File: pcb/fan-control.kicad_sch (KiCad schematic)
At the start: 23 parts, among them J1 USB_C_Receptacle_USB2.0_14P, J2 USB_C_Receptacle_USB2.0_14P, Q1 BSS138, SW1 SW_Push, U1 ESP32-C6-WROOM-1-N8

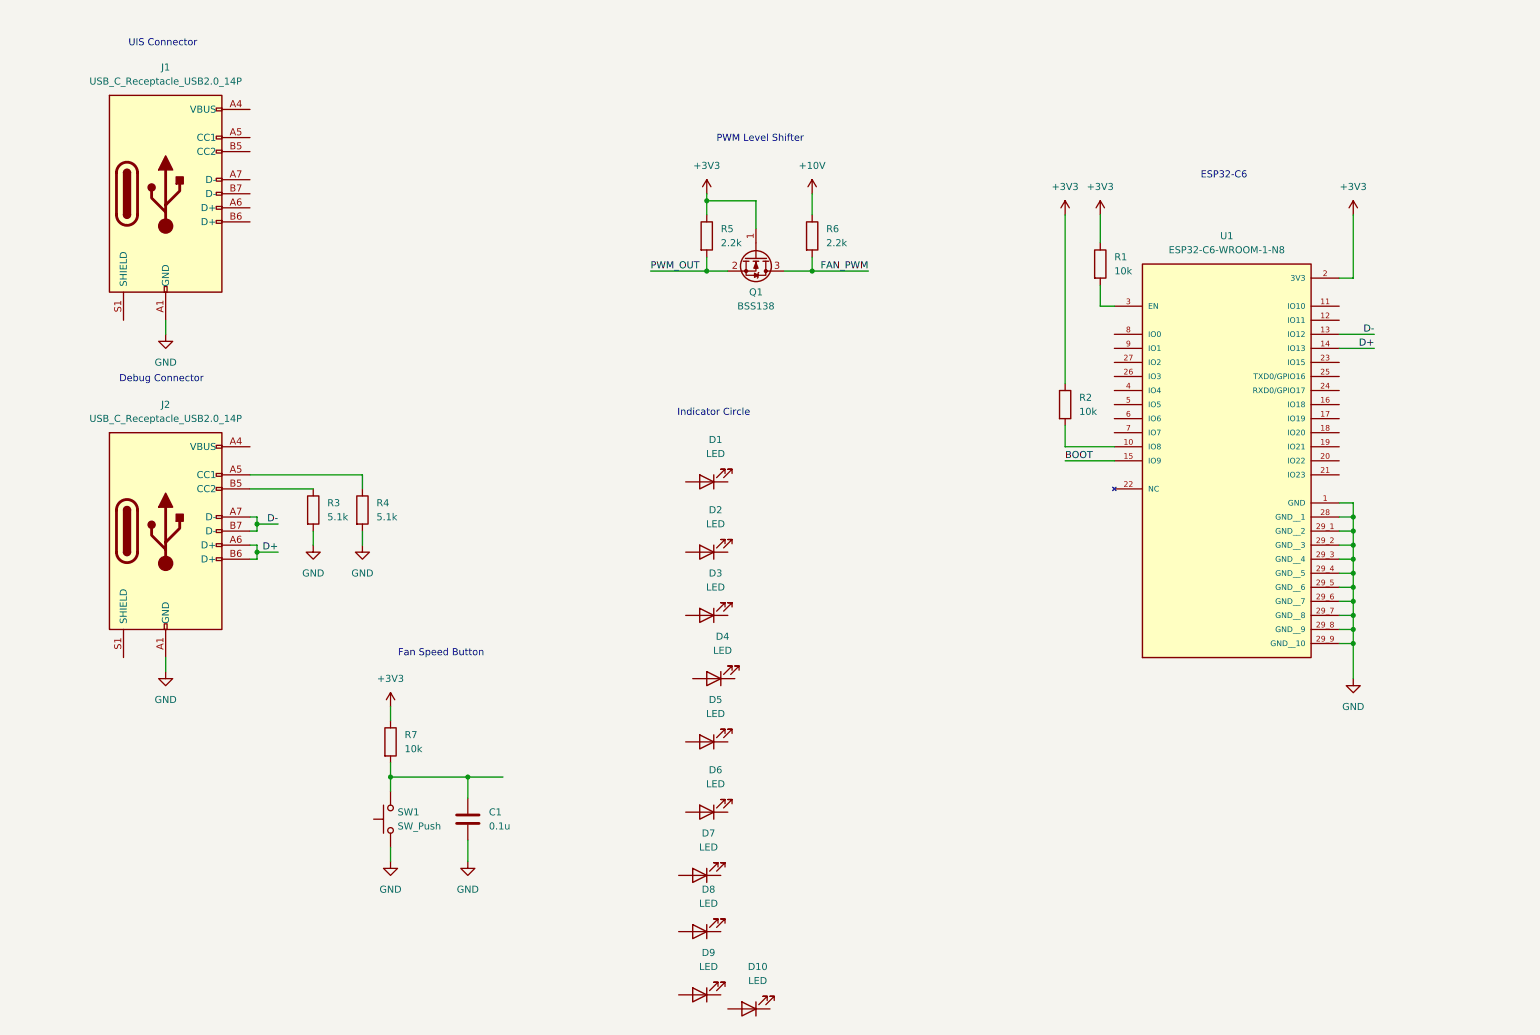
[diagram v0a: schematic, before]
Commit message: schematic
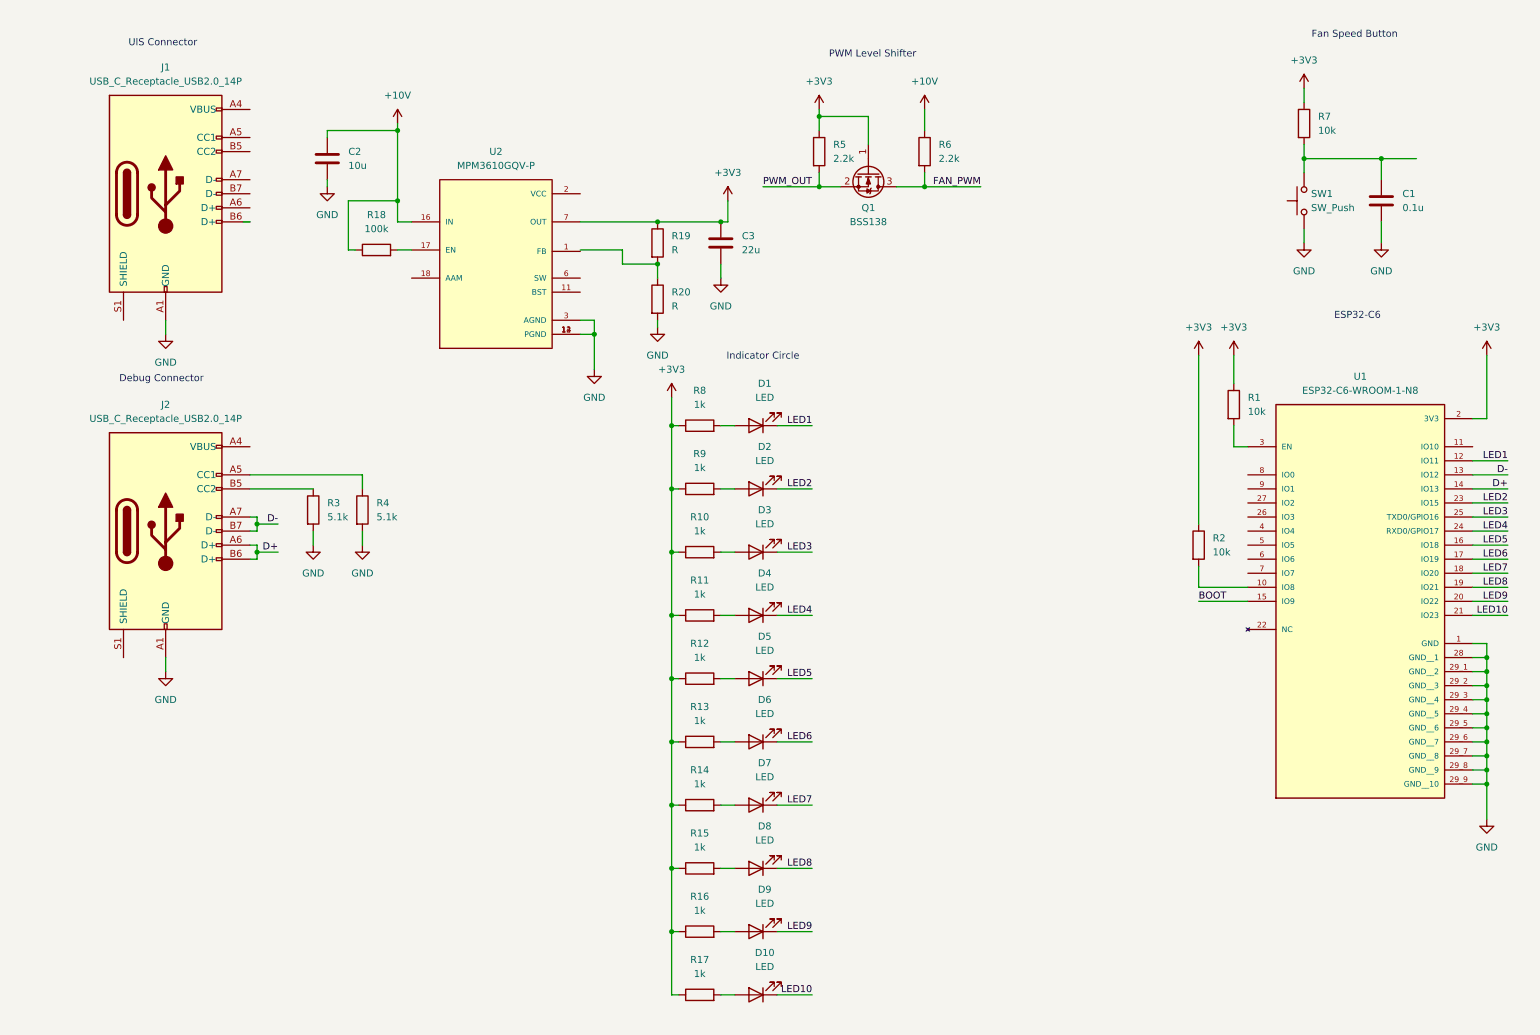
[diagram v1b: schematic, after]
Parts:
- added C2: 10u, symbol Device:C
- added C3: 22u, symbol Device:C
- added R10, R11, R12, R13, R14, R15, R16, R17, R8, R9: 1k, symbol Device:R
- added R18: 100k, symbol Device:R
- added R19, R20: R, symbol Device:R
- added U2: MPM3610GQV-P, MPM3610GQV-P:CONV_MPM3610GQV-P, symbol MPM3610GQV-P:MPM3610GQV-P
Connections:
- net +10V: now also C2.1, R18.1, U2.16 (IN)
- net +3V3: now also C3.1, R10.1, R11.1, R12.1, R13.1, R14.1, R15.1, R16.1, R17.1, R19.1, R8.1, R9.1, U2.7 (OUT)
- net GND: now also C2.2, C3.2, R20.2, U2.12 (PGND), U2.13 (PGND), U2.14 (PGND), U2.3 (AGND)
- net LED1: now reaches D1.1 (K)
- net LED1: now also U1.12 (IO11)
- net at D1.2 (A): now also R8.2
- net LED10: now reaches D10.1 (K)
- net LED10: now also U1.21 (IO23)
- net at D10.2 (A): now also R17.2
- net LED3: now reaches D3.1 (K)
- net LED3: now also U1.25 (TXD0/GPIO16)
- net at D3.2 (A): now also R10.2
- net LED7: now reaches D7.1 (K)
- net LED7: now also U1.18 (IO20)
- net at D7.2 (A): now also R14.2
- net LED8: now reaches D8.1 (K)
- net LED8: now also U1.19 (IO21)
- net at D8.2 (A): now also R15.2
- net LED5: now reaches U1.16 (IO18)
- net LED5: now also D5.1 (K)
- net LED6: now reaches U1.17 (IO19)
- net LED6: now also D6.1 (K)
- net LED9: now reaches U1.20 (IO22)
- net LED9: now also D9.1 (K)
- net LED2: now reaches U1.23 (IO15)
- net LED2: now also D2.1 (K)
- net LED4: now reaches U1.24 (RXD0/GPIO17)
- net LED4: now also D4.1 (K)
- net at D5.2 (A): now also R12.2
- net at D4.2 (A): now also R11.2
- net at D9.2 (A): now also R16.2
- net at D6.2 (A): now also R13.2
- net at D2.2 (A): now also R9.2
- new net: R18.2, U2.17 (EN)
- new net: R19.2, R20.1
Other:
- moved on the sheet: C1, D1, D10, D2, D3, D4, D5, D6, D7, D8, D9, Q1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

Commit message: More sch
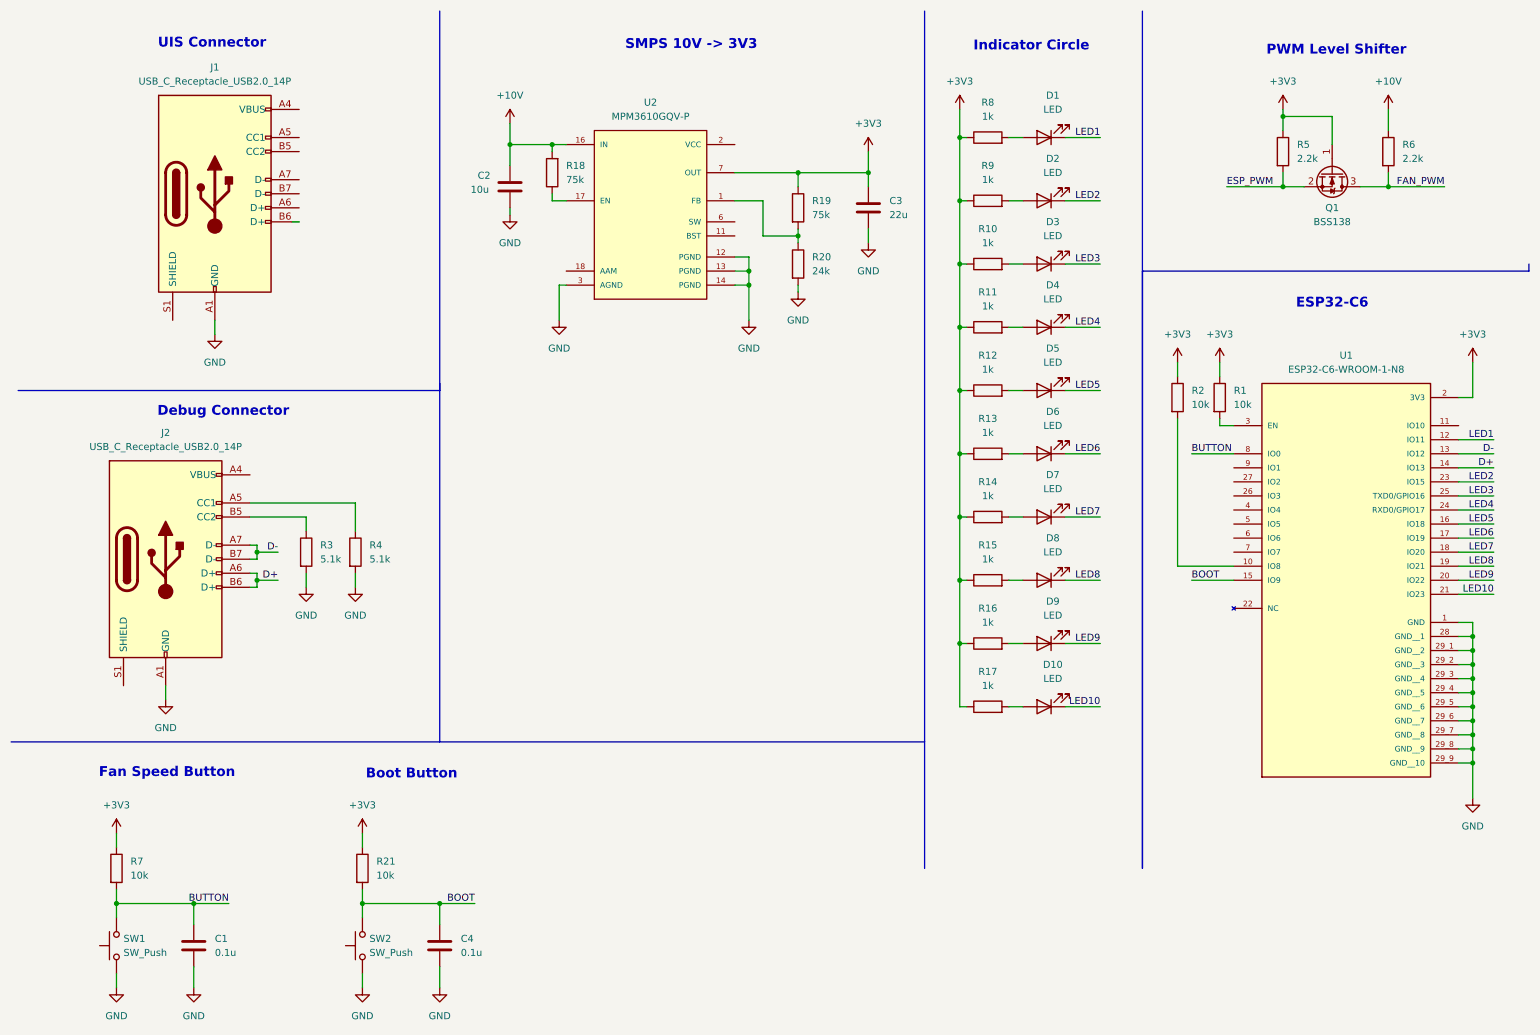
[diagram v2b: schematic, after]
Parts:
- added C4: 0.1u, symbol Device:C
- added R21: 10k, symbol Device:R
- added SW2: SW_Push, symbol Switch:SW_Push
- R18: value 100k -> 75k
- R19: value R -> 75k
- R20: value R -> 24k
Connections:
- net +10V: now also R18.2; no longer R18.1
- net +3V3: now also R21.1
- net BOOT: now also C4.1, R21.2, SW2.2
- net GND: now also C4.2, SW2.1
- net at U2.17 (EN): now also R18.1; no longer R18.2
- net BUTTON: now reaches U1.8 (IO0)
- net BUTTON: now also C1.1, R7.2, SW1.2
- net at R19.2, R20.1: now also U2.1 (FB)
- net PWM_OUT renamed ESP_PWM
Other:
- note added: "Boot Button"
- note added: "SMPS 10V -> 3V3"
- title: (none) -> UIS Fan Controller
- moved on the sheet: C1, C2, C3, D1, D10, D2, D3, D4, D5, D6, D7, D8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
